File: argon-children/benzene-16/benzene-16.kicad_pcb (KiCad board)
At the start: 2 copper layers, 25 x 25 mm, 20 parts, among them U1 Conn1, U2 SPI FLASH, U3 Conn2, U4 LMC555, U5 IS25WP256D-xM

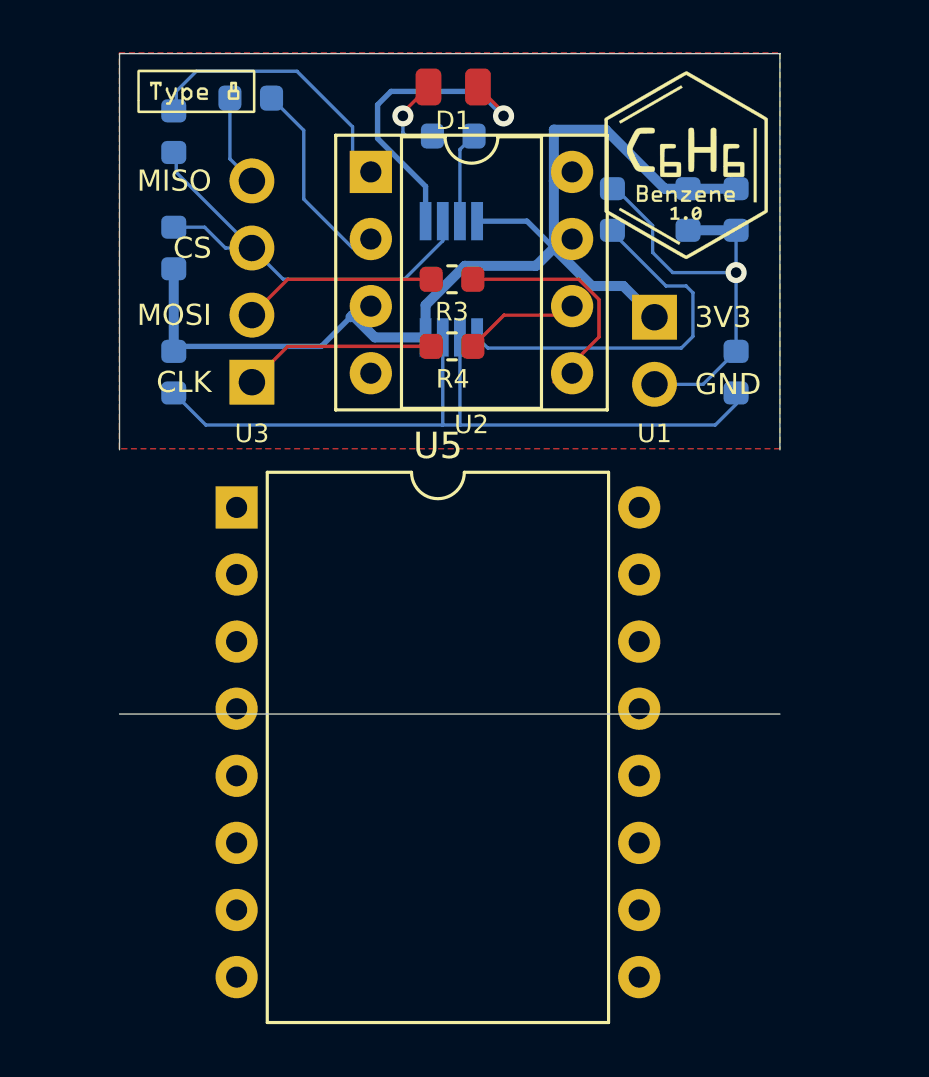
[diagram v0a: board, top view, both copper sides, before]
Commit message: Aegon USB and power
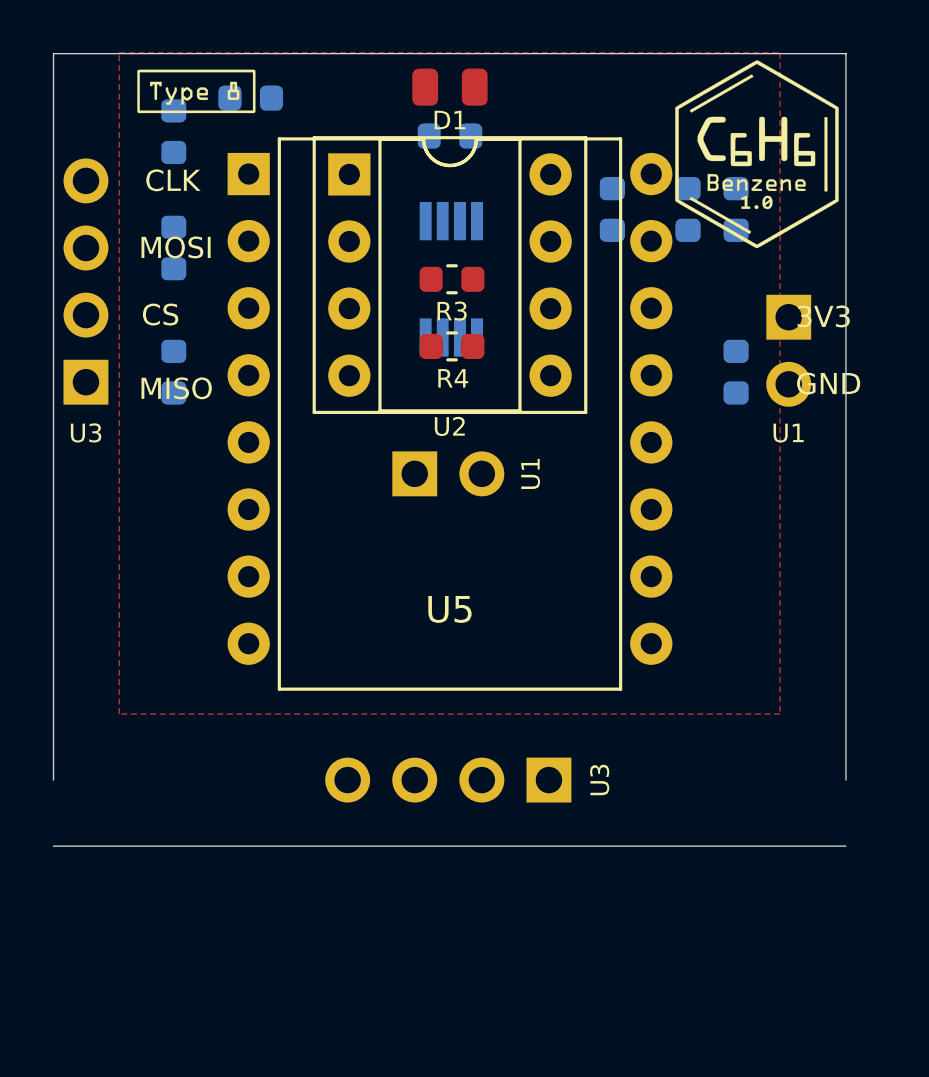
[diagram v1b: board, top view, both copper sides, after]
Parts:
- added U1: Conn1, Connector_PinHeader_2.54mm:PinHeader_1x02_P2.54mm_Vertical, B.Cu at (102.2, 83.9)
- added U3: Conn2, Connector_PinHeader_2.54mm:PinHeader_1x04_P2.54mm_Vertical, B.Cu at (107.3, 95.5)
- moved U5 12.6 mm to (95.9, 72.6)
- moved U3 6.28 mm to (89.7, 80.4)
- moved U1 5.08 mm to (116.3, 78.0)
- moved G*** 2.71 mm to (115.1, 71.8)
- moved U2 0.82 mm to (99.7, 72.6)
- moved D1 0.12 mm to (103.5, 69.3)
- moved R6 0.12 mm to (103.5, 71.1)
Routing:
- net V3V3: track 42.0 -> 0.00 mm
- net Net-(C4-Pad1): track 29.2 -> 0.00 mm
- net GND: track 28.8 -> 0.00 mm, vias 2 -> 0
- net ~CS: track 17.2 -> 0.00 mm
- net Net-(C3-Pad1): track 14.2 -> 0.00 mm
- net Net-(R2-Pad1): track 10.6 -> 0.00 mm
- net Net-(R3-Pad1): track 8.93 -> 0.00 mm
- net Net-(R4-Pad2): track 7.35 -> 0.00 mm
- net Net-(R3-Pad2): track 7.35 -> 0.00 mm
- net Net-(R1-Pad1): track 6.94 -> 0.00 mm
- net Net-(R4-Pad1): track 3.56 -> 0.00 mm
- net Net-(R1-Pad2): track 3.48 -> 0.00 mm
- net Net-(R6-Pad1): track 3.46 -> 0.00 mm
- net Net-(D1-Pad2): track 3.30 -> 0.00 mm, vias 1 -> 0
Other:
- board size 25 x 25 mm -> 30 x 30 mm
